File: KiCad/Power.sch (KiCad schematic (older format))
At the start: 59 parts, among them J3 Conn_IEC-320-C13_Socket, T1 373BX, T2 1650PA

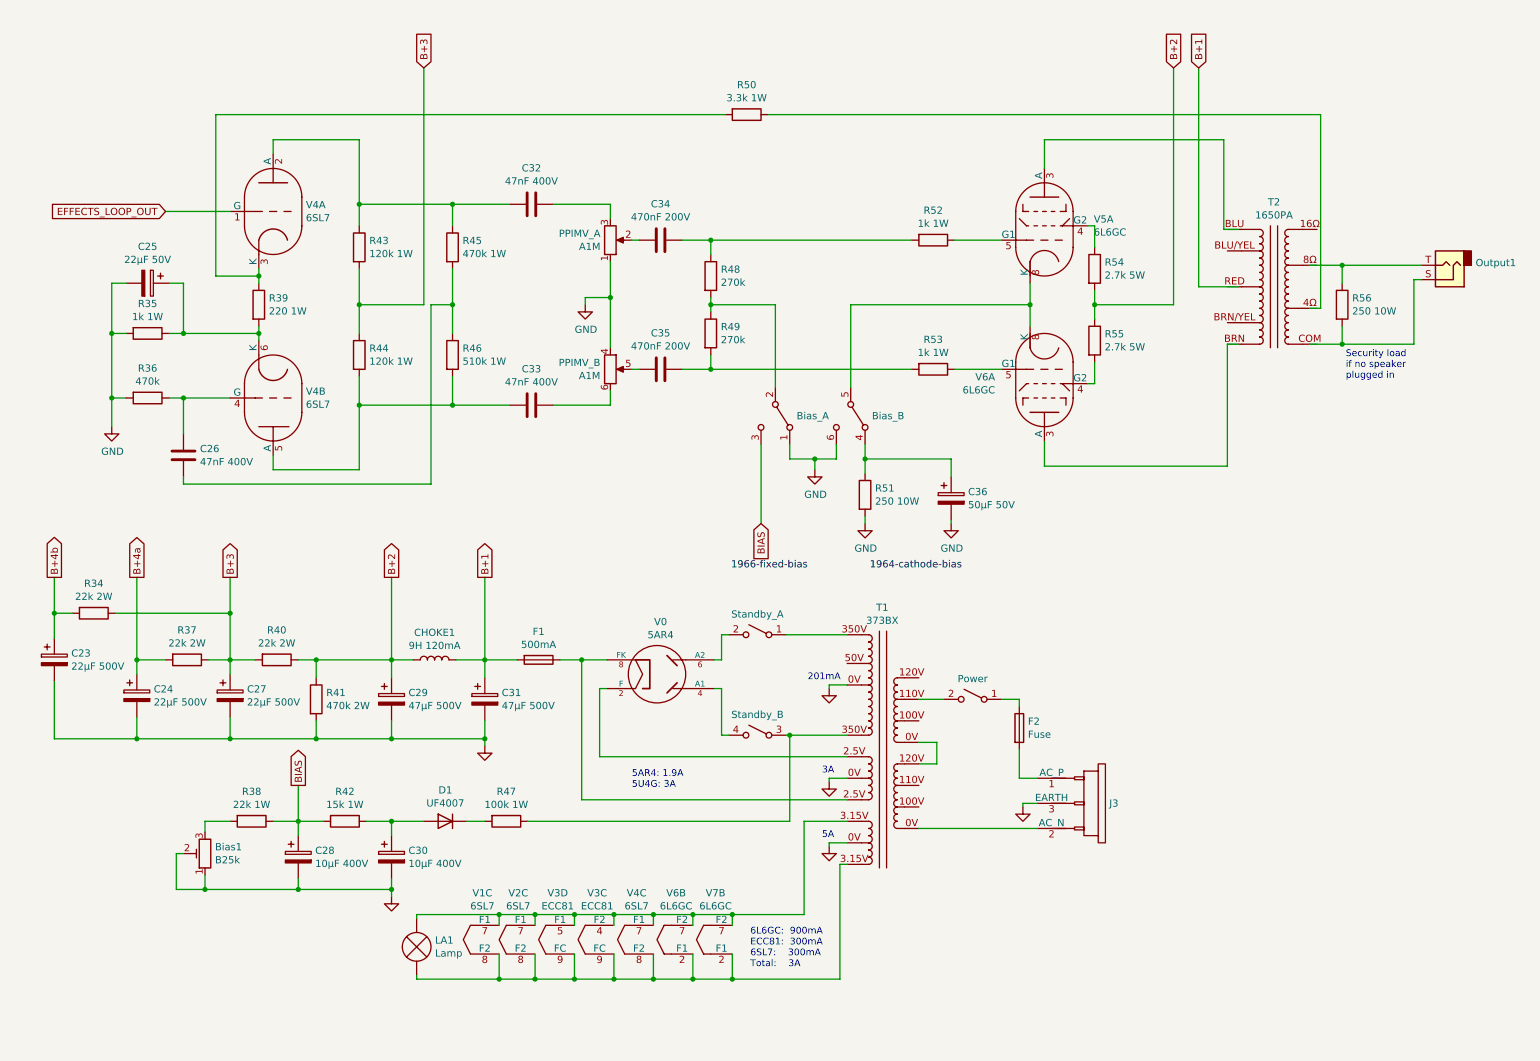
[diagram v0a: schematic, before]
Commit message: v2 before KiCad6 to rebase with the final commit
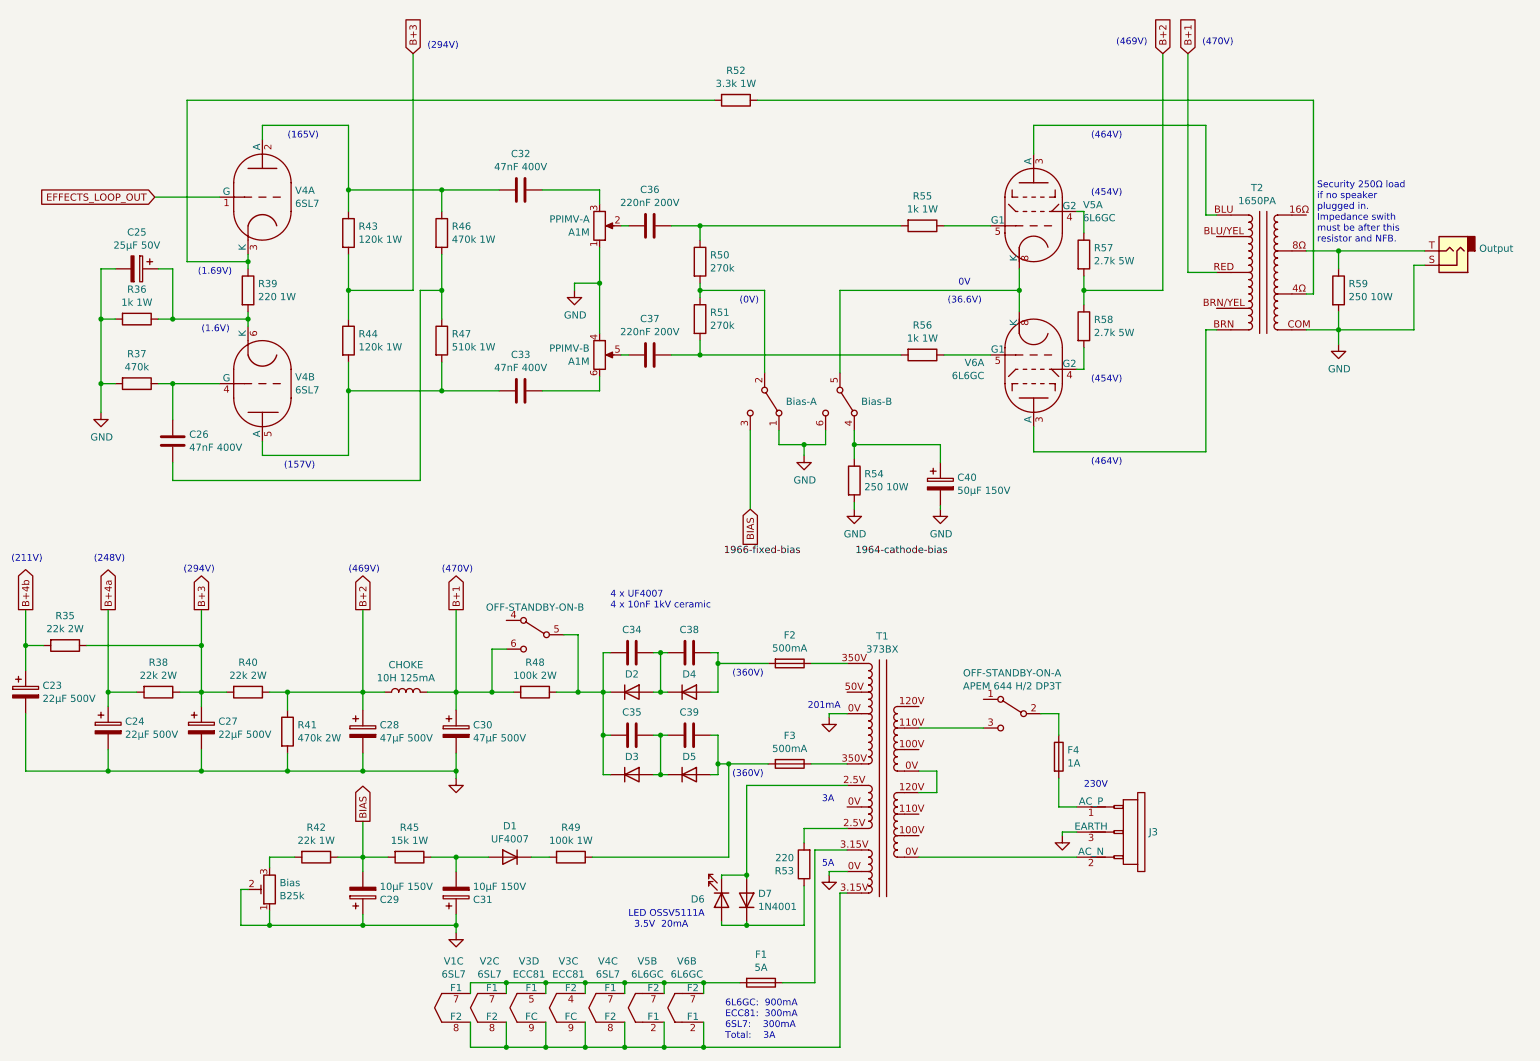
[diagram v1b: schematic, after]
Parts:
- removed LA1: Lamp, symbol Device:Lamp
- removed Power: SW_SPST, symbol Switch:SW_SPST
- removed Standby_: SW_DPST_x2, symbol Switch:SW_DPST_x2
- removed V0: 5AR4, Valve:Valve_Octal, symbol Vacuum_Tube:5AR4
- added C34, C35, C38, C39: 10nF 1kV, symbol Device:C
- added D2, D3, D4, D5: UF4007, Diode_THT:D_DO-41_SOD81_P10.16mm_Horizontal, symbol Diode:1N4007
- added D6: LED, symbol Device:LED
- added D7: 1N4001, Diode_THT:D_DO-41_SOD81_P10.16mm_Horizontal, symbol Diode:1N4007
- added F2, F3: 500mA, symbol Device:Fuse
- added OFF-STANDBY-ON-: APEM 644 H/2 DP3T, symbol Switch:SW_DPDT_x2
- added R48: 100k 2W, symbol Device:R
- added R53: 220, symbol Device:R
- C25: value 22µF 50V -> 25µF 50V
- C29: renamed from C28; value 10µF 400V -> 10µF 150V
- C31: renamed from C30; value 10µF 400V -> 10µF 150V
- C36: renamed from C34; value 470nF 200V -> 220nF 200V
- C37: renamed from C35; value 470nF 200V -> 220nF 200V
- C40: renamed from C36; value 50µF 50V -> 50µF 150V
- CHOKE: renamed from CHOKE1; value 9H 120mA -> 10H 125mA
- F1: value 500mA -> 5A
- F4: renamed from F2; value Fuse -> 1A
- renumbered Bias1 to Bias, Bias_ to Bias-, C29 to C28, C31 to C30, Output1 to Output, PPIMV_ to PPIMV-, R34 to R35, R35 to R36, R36 to R37, R37 to R38, R38 to R42, R42 to R45, R45 to R46, R46 to R47, R47 to R49, R48 to R50, R49 to R51, R50 to R52, R51 to R54, R52 to R55, R53 to R56, R54 to R57, R55 to R58, R56 to R59, V6 to V5, V7 to V6
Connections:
- wire segments 236 -> 265
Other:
- note added: "(0V)"
- note added: "(1.69V)"
- note added: "(1.6V)"
- note added: "(157V)"
- note added: "(165V)"
- note added: "(211V)"
- note added: "(248V)"
- note added: "(294V)"
- note added: "(36.6V)"
- note added: "(360V)"
- note added: "(454V)"
- note added: "(464V)"
- note added: "(469V)"
- note added: "(470V)"
- note added: "0V"
- note added: "230V"
- note added: "4 x UF4007\n4 x 10nF 1kV ceramic"
- note added: "LED OSSV5111A\n 3.5V 20mA"
- note added: "Security 250Ω load\nif no speaker\nplugged in.\nImpedance swith\nmust be after this\nresistor and NFB."
- note removed: "5AR4: 1.9A\n5U4G: 3A"
- note removed: "Security load\nif no speaker\nplugged in"
- moved on the sheet: Bias, Bias-A, Bias-B, C23, C24, C25, C26, C27, C28, C29, C30, C31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
